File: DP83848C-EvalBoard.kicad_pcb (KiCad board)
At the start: 4 copper layers, 100 x 100 mm, 173 parts, among them J1 Conn_02x08_Odd_Even, J10 RJ45_LED_Shielded, J11 USB_C_Receptacle_USB2.0, J12 Conn_02x05_Odd_Even, J13 Conn_01x04, J14 Conn_02x04_Odd_Even, J2 Conn_02x08_Odd_Even, J3 Conn_02x04_Odd_Even, J4 Conn_01x04, J5 Conn_01x04, J6 Conn_02x04_Odd_Even, J7 Conn_02x04_Odd_Even, J8 Conn_02x04_Odd_Even, J9 Conn_01x02, Q1 AO3401A, Q2 AO3400A, Q3 AO3401A, SW1 SW_Push, T1 H1102NL, U1 AMS1117-3.3, U2 DP83848C, U3 STM32F407VGTx, U4 USBLC6-2SC6, X1 50MHz, Y1 25MHz

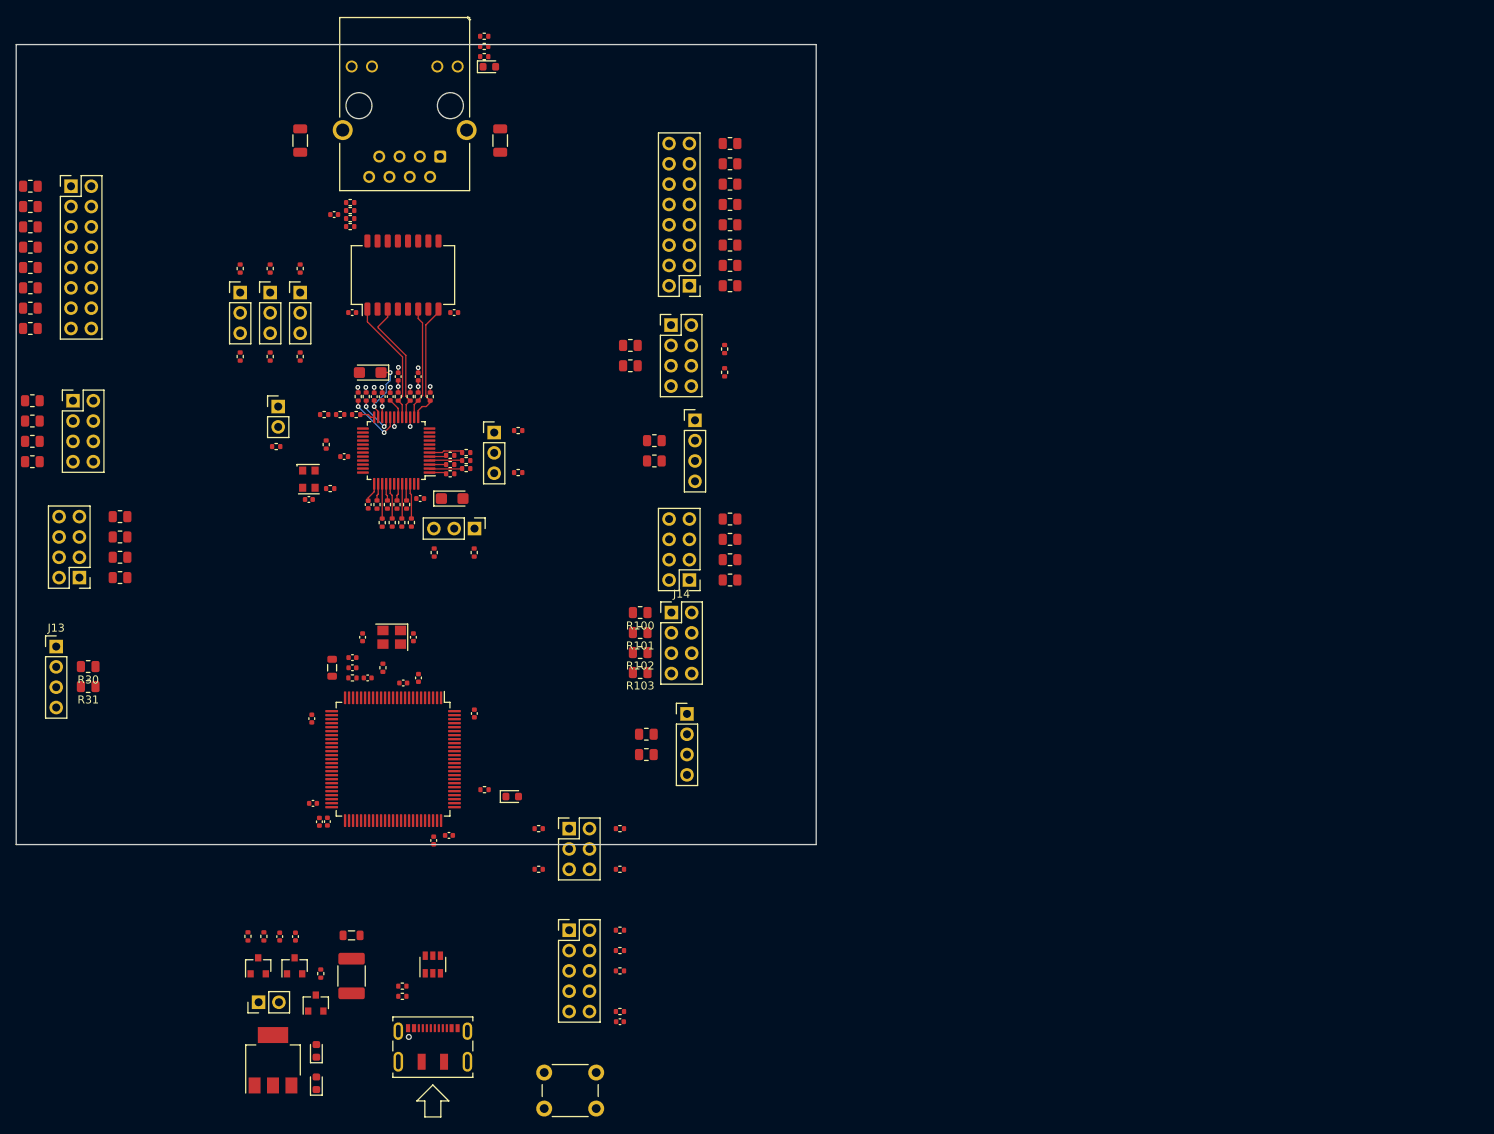
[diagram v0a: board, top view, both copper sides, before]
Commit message: Routing
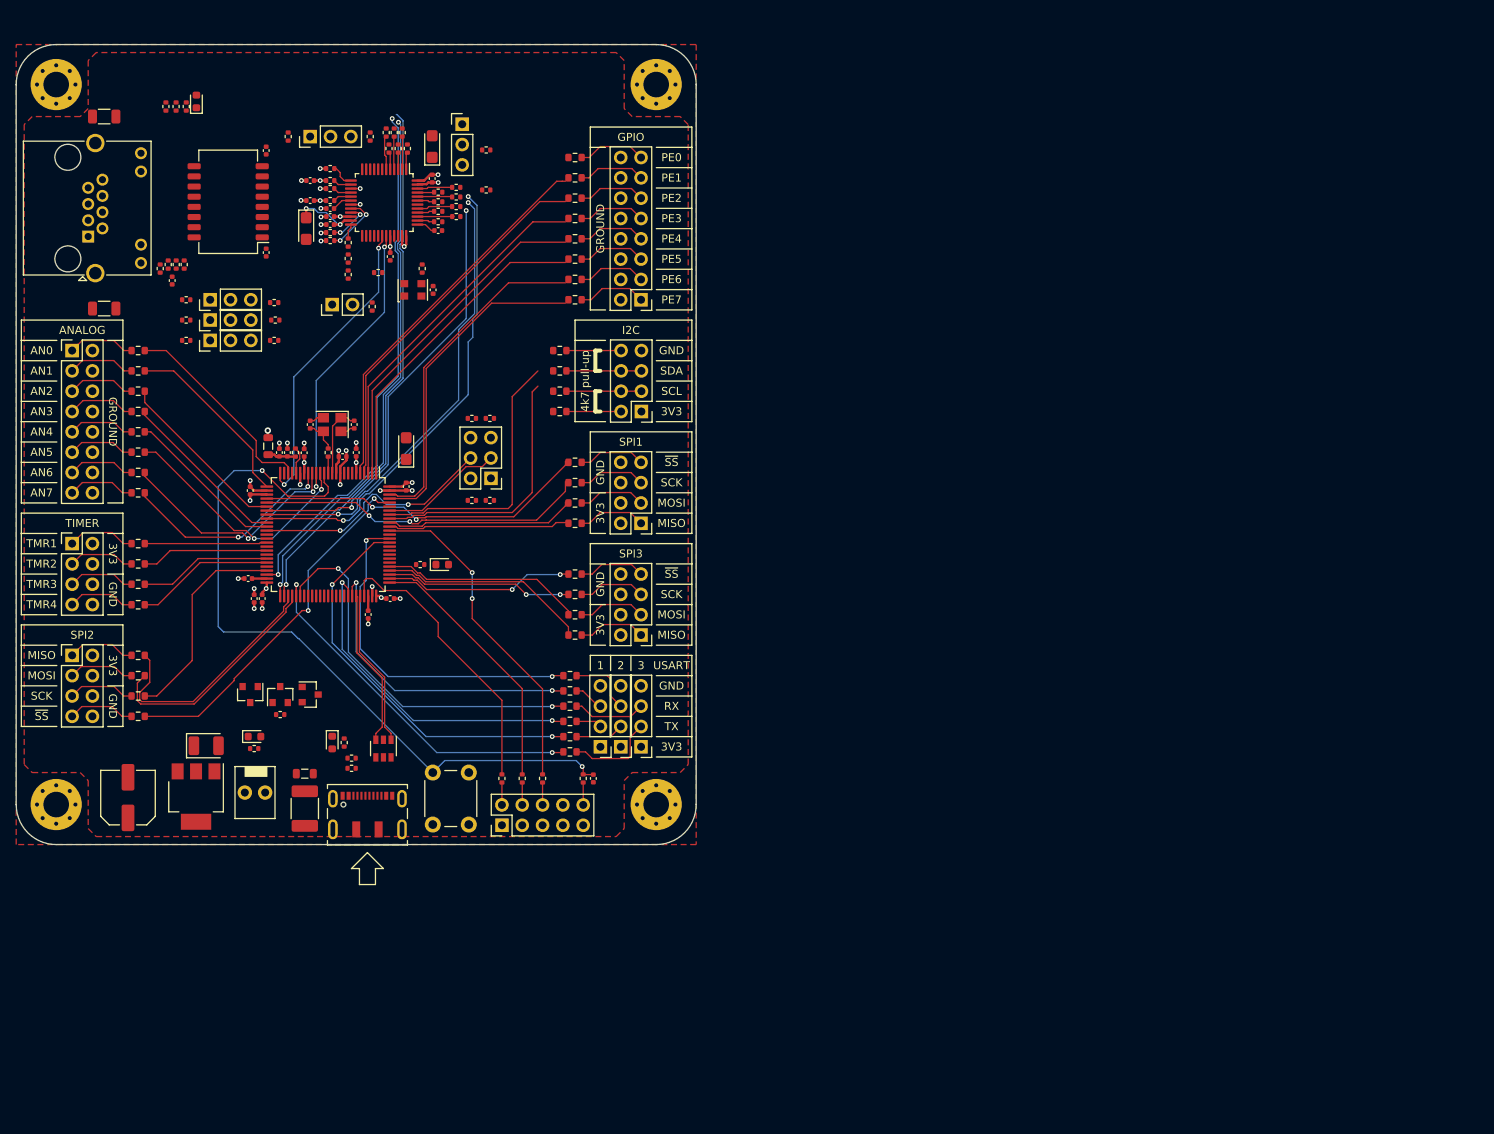
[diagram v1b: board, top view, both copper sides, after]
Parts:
- added C32: 10uF, Capacitor_Tantalum_SMD:CP_EIA-3216-18_Kemet-A, F.Cu at (88.8, 107.5)
- added H1: MountingHole_Pad, MountingHole:MountingHole_3.2mm_M3_Pad_Via, F.Cu at (45.0, 152.0)
- added H2: MountingHole_Pad, MountingHole:MountingHole_3.2mm_M3_Pad_Via, F.Cu at (45.0, 62.0)
- added H3: MountingHole_Pad, MountingHole:MountingHole_3.2mm_M3_Pad_Via, F.Cu at (120.0, 152.0)
- added H4: MountingHole_Pad, MountingHole:MountingHole_3.2mm_M3_Pad_Via, F.Cu at (120.0, 62.0)
- C1: footprint Capacitor_SMD:C_0402_1005Metric -> Capacitor_SMD:C_Elec_6.3x7.7
- C2: value 22uF -> 100uF; footprint Capacitor_SMD:C_0402_1005Metric -> Capacitor_Tantalum_SMD:CP_EIA-3528-15_AVX-H
- J10: footprint Connector_RJ:RJ45_Hanrun_HR911105A -> Connector_RJ:RJ45_Amphenol_RJHSE538X
- J9: footprint Connector_PinHeader_2.54mm:PinHeader_1x02_P2.54mm_Vertical -> ak:Molex_022112022
- R1, R2: footprint Resistor_SMD:R_0402_1005Metric -> Resistor_SMD:R_0603_1608Metric
- R100, R101, R102, R103, R30, R31, R64, R65, R66, R67, R68, R69, R70, R71, R72, R73, R74, R75, R76, R77, R78, R79, R80, R81, R82, R83, R84, R85, R86, R87, R88, R89, R90, R91, R92, R93, R94, R95, R96, R97: footprint Resistor_SMD:R_0805_2012Metric -> Resistor_SMD:R_0603_1608Metric
- moved J13 74.2 mm to (118.1, 144.8), turned to 180 degrees
- moved R30 61.2 mm to (109.2, 145.4), turned to 0 degrees
- moved R31 60.3 mm to (109.2, 139.7), turned to 0 degrees
- moved R56 59.3 mm to (97.0, 103.7)
- moved R54 56.7 mm to (99.2, 103.7)
- moved JP2 50.6 mm to (95.8, 67.0), turned to 0 degrees
- moved R34 50.3 mm to (98.8, 70.2), turned to 180 degrees
- moved R98 49.6 mm to (51.0, 66.0), turned to 180 degrees
- moved R36 46.7 mm to (74.0, 68.5), turned to 90 degrees
- moved R37 45.9 mm to (84.2, 68.5), turned to 90 degrees
- moved R35 45.8 mm to (98.8, 75.2), turned to 180 degrees
- moved J10 45.1 mm to (49.0, 81.0), turned to 90 degrees
- moved R55 45.0 mm to (97.0, 114.0)
- moved JP7 44.9 mm to (99.3, 111.2), turned to 180 degrees
- moved C4 44.1 mm to (92.0, 69.8), turned to 90 degrees
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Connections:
- net /ADC0 renamed /MCU/ADC_IN0
- net /ADC1 renamed /MCU/ADC_IN3
- net /ADC2 renamed /MCU/ADC_IN6
- net /ADC3 renamed /MCU/ADC_IN8
- net /ADC4 renamed /MCU/ADC_IN9
- net /ADC5 renamed /MCU/ADC_IN10
- net /ADC6 renamed /MCU/ADC_IN12
- net /ADC7 renamed /MCU/ADC_IN13
- net /GPIO0 renamed /MCU/GPIO0
- net /GPIO1 renamed /MCU/GPIO1
- net /GPIO2 renamed /MCU/GPIO2
- net /GPIO3 renamed /MCU/GPIO3
- net /GPIO4 renamed /MCU/GPIO4
- net /GPIO5 renamed /MCU/GPIO5
- net /GPIO6 renamed /MCU/GPIO6
- net /GPIO7 renamed /MCU/GPIO7
- net /TMR1 renamed /MCU/TMR_CH1
- net /TMR2 renamed /MCU/TMR_CH2
- net /TMR3 renamed /MCU/TMR_CH3
- net /TMR4 renamed /MCU/TMR_CH4
- net Net-(J1-Pad1) renamed /GPIO0_R
- net Net-(J1-Pad11) renamed /GPIO5_R
- net Net-(J1-Pad13) renamed /GPIO6_R
- net Net-(J1-Pad15) renamed /GPIO7_R
- net Net-(J1-Pad3) renamed /GPIO1_R
- net Net-(J1-Pad5) renamed /GPIO2_R
- net Net-(J1-Pad7) renamed /GPIO3_R
- net Net-(J1-Pad9) renamed /GPIO4_R
- net Net-(J13-Pad2) renamed /USART3_TX_R
- net Net-(J13-Pad3) renamed /USART3_RX_R
- net Net-(J14-Pad1) renamed /SPI3_MISO_R
- net Net-(J14-Pad3) renamed /SPI3_MOSI_R
- net Net-(J14-Pad5) renamed /SPI3_SCK_R
- net Net-(J14-Pad7) renamed /SPI3_NSS_R
- net Net-(J2-Pad1) renamed /ADC0_R
- net Net-(J2-Pad11) renamed /ADC5_R
- net Net-(J2-Pad13) renamed /ADC6_R
- net Net-(J2-Pad15) renamed /ADC7_R
- net Net-(J2-Pad3) renamed /ADC1_R
- net Net-(J2-Pad5) renamed /ADC2_R
- net Net-(J2-Pad7) renamed /ADC3_R
- net Net-(J2-Pad9) renamed /ADC4_R
- net Net-(J3-Pad1) renamed /TMR1_R
- net Net-(J3-Pad3) renamed /TMR2_R
- net Net-(J3-Pad5) renamed /TMR3_R
- net Net-(J3-Pad7) renamed /TMR4_R
- net Net-(J4-Pad2) renamed /USART1_TX_R
- net Net-(J4-Pad3) renamed /USART1_RX_R
- net Net-(J5-Pad2) renamed /USART2_TX_R
- net Net-(J5-Pad3) renamed /USART2_RX_R
- net Net-(J6-Pad1) renamed /SPI1_MISO_R
- net Net-(J6-Pad3) renamed /SPI1_MOSI_R
- net Net-(J6-Pad5) renamed /SPI1_SCK_R
- net Net-(J6-Pad7) renamed /SPI1_NSS
- net Net-(J7-Pad1) renamed /SPI2_MISO_R
- net Net-(J7-Pad3) renamed /SPI2_MOSI_R
- net Net-(J7-Pad5) renamed /SPI2_SCK_R
- net Net-(J7-Pad7) renamed /SPI2_NSS_R
- net Net-(R51-Pad1) renamed /MCU/VREF+
- J8 pad 2: +3V3 -> Net-(J8-Pad2)
- J8 pad 3: Net-(J8-Pad3) -> /I2C1_SCL_R
- J8 pad 4: Net-(J8-Pad4) -> /I2C1_SCL_R
- J8 pad 5: Net-(J8-Pad5) -> /I2C1_SDA_R
- J8 pad 6: Net-(J8-Pad6) -> /I2C1_SDA_R
- J8 pad 8: +3V3 -> Net-(J8-Pad8)
- R1 pad 1: Net-(J8-Pad6) -> +3V3
- R1 pad 2: Net-(J8-Pad5) -> Net-(J8-Pad2)
- R2 pad 1: Net-(J8-Pad4) -> +3V3
- R2 pad 2: Net-(J8-Pad3) -> Net-(J8-Pad8)
- R30 pad 1: /MCU/USART3_RX -> /MCU/USART3_TX
- R31 pad 1: /MCU/USART3_TX -> /MCU/USART3_RX
- R84 pad 1: /USART1_RX -> /MCU/USART1_TX
- R85 pad 1: /USART1_TX -> /MCU/USART1_RX
- R86 pad 1: /USART2_RX -> /MCU/USART2_TX
- R87 pad 1: /USART2_TX -> /MCU/USART2_RX
- R96 pad 1: Net-(J8-Pad3) -> /I2C1_SCL_R
- R96 pad 2: /MCU/I2C1_SDA -> /MCU/I2C1_SCL
- R97 pad 1: Net-(J8-Pad5) -> /I2C1_SDA_R
- R97 pad 2: /MCU/I2C1_SCL -> /MCU/I2C1_SDA
- U3 pad 68: /USART1_TX -> /MCU/USART1_TX
- U3 pad 69: /USART1_RX -> /MCU/USART1_RX
- U3 pad 86: /USART2_TX -> /MCU/USART2_TX
- U3 pad 87: /USART2_RX -> /MCU/USART2_RX
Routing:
- net /MCU/NRST: track 0.00 -> 92.5 mm, vias 0 -> 2
- net /ETH_TX_D1: track 0.00 -> 67.3 mm, vias 0 -> 1
- net /ETH_TX_D0: track 0.00 -> 66.4 mm, vias 0 -> 2
- net /ETH_TX_EN: track 0.00 -> 66.0 mm, vias 0 -> 2
- net /ETH_RXD1: track 0.00 -> 58.2 mm, vias 0 -> 2
- net /ETH_RXD0: track 0.00 -> 56.4 mm, vias 0 -> 2
- net /ETH_CRS_DV: track 0.00 -> 53.8 mm, vias 0 -> 2
- net /MCU/USART2_TX: track 0.00 -> 50.4 mm, vias 0 -> 2
- net /MCU/GPIO6: track 0.00 -> 47.8 mm
- net /MCU/USART3_RX: track 0.00 -> 47.5 mm, vias 0 -> 2
- net /MCU/GPIO5: track 0.00 -> 46.2 mm
- net /MCU/SPI2_NSS: track 0.00 -> 45.6 mm, vias 0 -> 2
- net /MCU/USART3_TX: track 0.00 -> 45.6 mm, vias 0 -> 2
- net /MCU/GPIO4: track 0.00 -> 44.0 mm
- net /MCU/USART2_RX: track 0.00 -> 43.7 mm, vias 0 -> 2
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- added copper zone on In2.Cu, net +3V3
- added copper zone on In1.Cu, net GND
- added copper zone on F.Cu, net GNDPWR
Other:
- board size 100 x 100 mm -> 85 x 100 mm
- board text added: "1"
- board text added: "2"
- board text added: "3"
- board text added: "3V3"
- board text added: "4k7 pull-up"
- board text added: "AN0"
- board text added: "AN1"
- board text added: "AN2"
- board text added: "AN3"
- board text added: "AN4"
- board text added: "AN5"
- board text added: "AN6"
- board text added: "AN7"
- board text added: "ANALOG"
- board text added: "GND"
- board text added: "GPIO"
- board text added: "GROUND"
- board text added: "I2C"
- board text added: "MISO"
- board text added: "MOSI"
- board text added: "PE0"
- board text added: "PE1"
- board text added: "PE2"
- board text added: "PE3"
- board text added: "PE4"
- board text added: "PE5"
- board text added: "PE6"
- board text added: "PE7"
- board text added: "RX"
- board text added: "SCK"
- board text added: "SCL"
- board text added: "SDA"
- board text added: "SPI1"
- board text added: "SPI2"
- board text added: "SPI3"
- board text added: "TIMER"
- board text added: "TMR1"
- board text added: "TMR2"
- board text added: "TMR3"
- board text added: "TMR4"
- board text added: "TX"
- board text added: "USART"
- board text added: "~SS"

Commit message: Layout
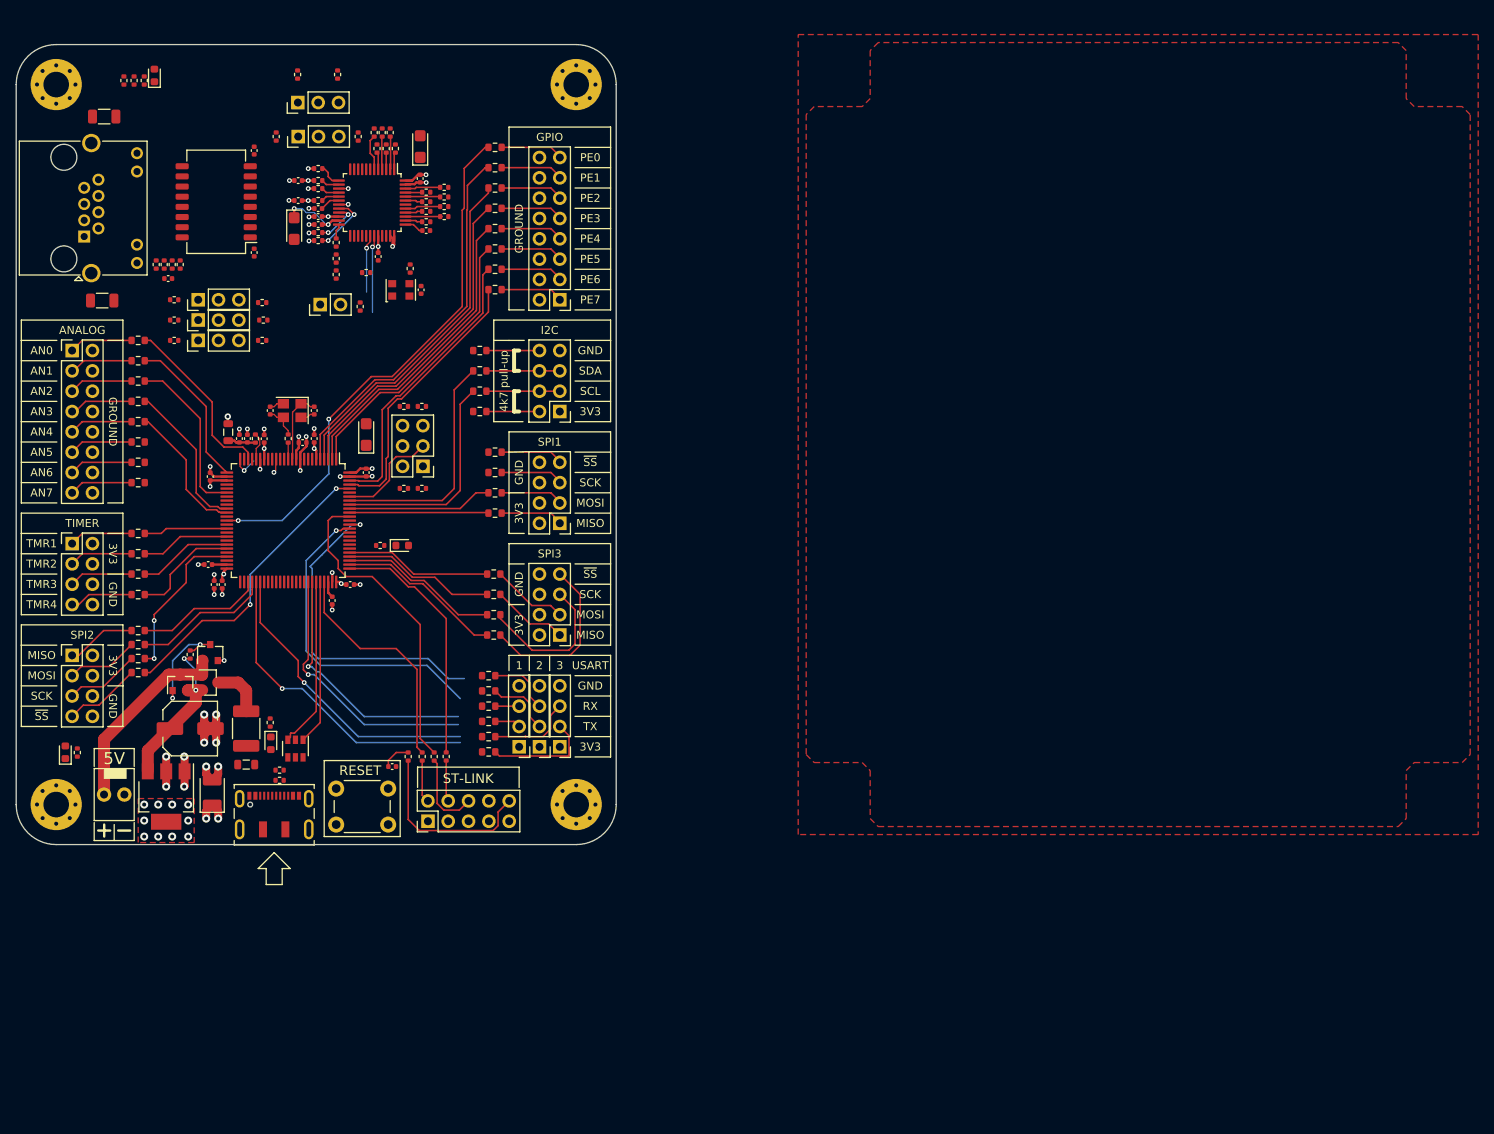
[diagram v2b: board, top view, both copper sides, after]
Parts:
- moved R34 25.4 mm to (75.2, 60.8), turned to 270 degrees
- moved C19 25.2 mm to (87.0, 147.2), turned to 0 degrees
- moved D1 23.7 mm to (46.1, 145.5), turned to 90 degrees
- moved R35 23.5 mm to (80.2, 60.8), turned to 270 degrees
- moved R3 22.1 mm to (47.6, 145.5), turned to 90 degrees
- moved R63 22.0 mm to (89.0, 146.0)
- moved JP2 20.7 mm to (75.2, 64.2), turned to 90 degrees
- moved J9 17.6 mm to (52.2, 150.8)
- moved R62 13.8 mm to (92.2, 146.0)
- moved R4 13.5 mm to (61.8, 133.2), turned to 90 degrees
- moved SW1 12.9 mm to (80.0, 150.0), turned to 0 degrees
- moved R103 12.7 mm to (99.7, 130.8)
- moved Q1 12.6 mm to (60.5, 136.8)
- moved Q3 12.6 mm to (64.2, 136.8)
- moved F1 12.4 mm to (68.8, 142.5), turned to 270 degrees
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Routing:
- net /MCU/NRST: track 92.5 -> 3.66 mm, vias 2 -> 0
- net /ETH_TX_D1: track 67.3 -> 0.00 mm, vias 1 -> 0
- net /ETH_TX_D0: track 66.4 -> 0.00 mm, vias 2 -> 0
- net /MCU/GPIO7: track 0.00 -> 66.0 mm, vias 0 -> 2
- net /ETH_TX_EN: track 66.0 -> 0.00 mm, vias 2 -> 0
- net /ETH_RXD1: track 58.2 -> 0.00 mm, vias 2 -> 0
- net /ETH_RXD0: track 56.4 -> 0.00 mm, vias 2 -> 0
- net /ETH_CRS_DV: track 53.8 -> 0.00 mm, vias 2 -> 0
- net /MCU/SPI1_NSS: track 41.7 -> 0.00 mm, vias 2 -> 0
- net /MCU/SPI1_SCK: track 41.3 -> 0.00 mm, vias 2 -> 0
- net /MCU/ADC_IN10: track 31.2 -> 0.00 mm, vias 2 -> 0
- net /MCU/BOOT1: track 30.8 -> 0.00 mm, vias 2 -> 0
- net /MCU/ADC_IN12: track 29.6 -> 0.00 mm, vias 2 -> 0
- net /MCU/ADC_IN13: track 27.3 -> 0.00 mm, vias 2 -> 0
- net /ETH_MDIO: track 37.8 -> 10.6 mm
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- added copper zone on F.Cu, net +3V3
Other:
- board size 85 x 100 mm -> 75 x 100 mm
- net class Default: clearance 0.15 -> 0.2; trace_width 0.15 -> 0.2
- net class Power added: clearance 0.2, trace_width 0.3, via_dia 0.6, via_drill 0.3
- rule trace_clearance: 0.15 -> 0.2
- board text added: "5V"
- board text added: "RESET"
- board text added: "ST-LINK"
